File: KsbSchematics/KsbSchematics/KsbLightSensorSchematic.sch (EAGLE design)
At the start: 29 parts, among them IC1 7805L, IC2 LM311N, U1 ATTINY84

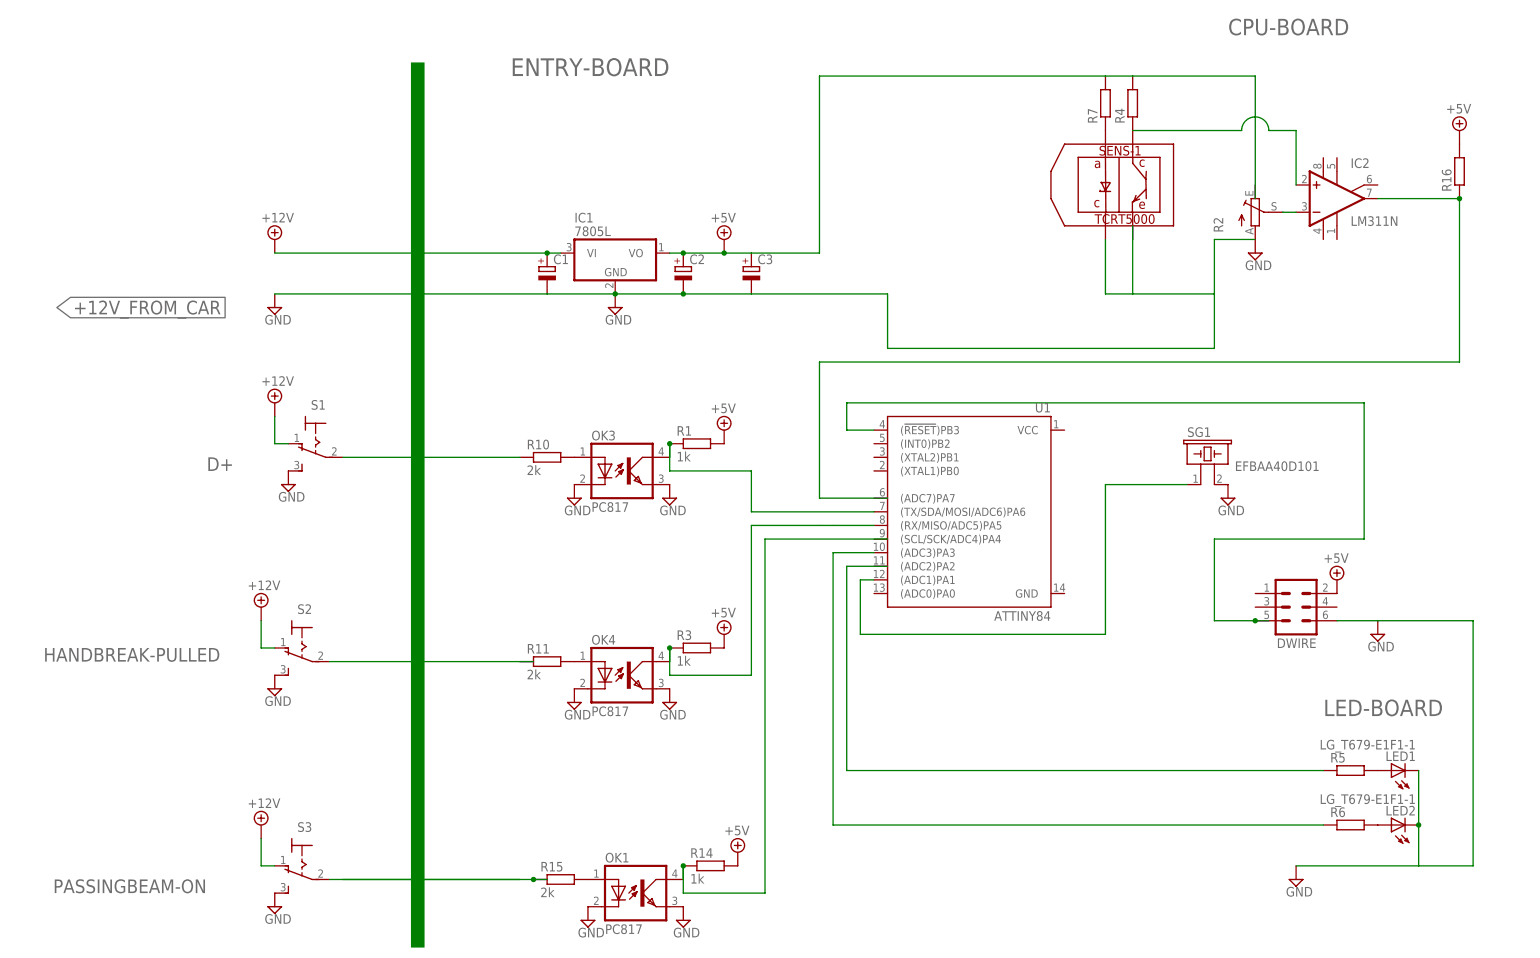
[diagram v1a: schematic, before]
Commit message: schematic changes
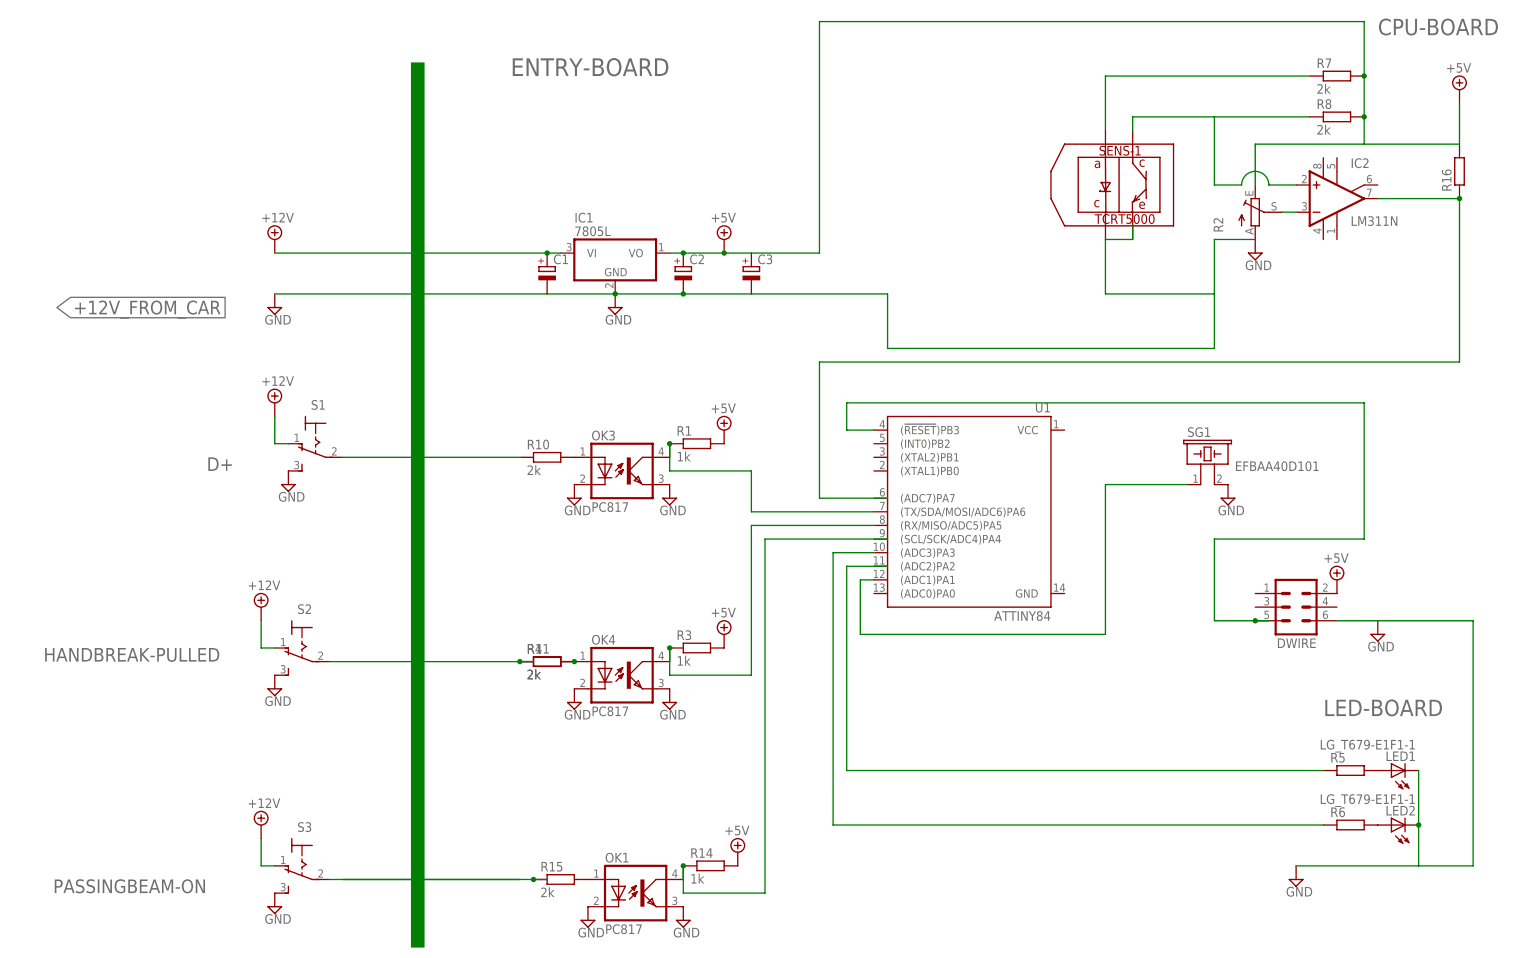
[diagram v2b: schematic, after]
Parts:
- added R8: 2k, resistor:R-EU_0613/5V
- R4, R7: value (none) -> 2k
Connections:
- net +12V: no longer R16.2
- net CPU-BOARD: now also IC2.OUT, R16.1; no longer IC2.+IN, SENS-1.P$1
- net ENTRY-BOARD: now also R16.2, R2.E, R8.2; no longer R4.2
- net N$1: now also R4.2
- net N$4: now also IC2.+IN, R8.1, SENS-1.P$1; no longer IC2.OUT, R16.1
- net PASSINGBEAM-ON: now also R4.1
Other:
- moved on the sheet: R4, R7
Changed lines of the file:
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@@
 <part name="R6" library="resistor" deviceset="R-EU_" device="0613/5V"/>
 <part name="SUPPLY17" library="supply2" deviceset="GND" device=""/>
-<part name="R4" library="resistor" deviceset="R-EU_" device="0613/5V"/>
-<part name="R7" library="resistor" deviceset="R-EU_" device="0613/5V"/>
 <part name="R10" library="resistor" deviceset="R-EU_" device="0613/5V" value="2k"/>
 <part name="R11" library="resistor" deviceset="R-EU_" device="0613/5V" value="2k"/>
@@
 <part name="DWIRE" library="con-lstb" deviceset="MA03-2" device=""/>
 <part name="SUPPLY25" library="supply2" deviceset="GND" device=""/>
+<part name="R4" library="resistor" deviceset="R-EU_" device="0613/5V" value="2k"/>
+<part name="R7" library="resistor" deviceset="R-EU_" device="0613/5V" value="2k"/>
+<part name="R8" library="resistor" deviceset="R-EU_" device="0613/5V" value="2k"/>
 </parts>
 <sheets>
@@
 <instance part="R6" gate="G$1" x="134.62" y="17.78"/>
 <instance part="SUPPLY17" gate="GND" x="111.76" y="78.74"/>
-<instance part="R4" gate="G$1" x="93.98" y="152.4" rot="R90"/>
-<instance part="R7" gate="G$1" x="88.9" y="152.4" rot="R90"/>
 <instance part="R10" gate="G$1" x="-15.24" y="86.36"/>
 <instance part="R11" gate="G$1" x="-15.24" y="48.26"/>
@@
 <instance part="R15" gate="G$1" x="-12.7" y="7.62"/>
 <instance part="R16" gate="G$1" x="154.94" y="139.7" rot="R90"/>
-<instance part="SUPPLY22" gate="+12V" x="154.94" y="147.32"/>
+<instance part="SUPPLY22" gate="+12V" x="154.94" y="154.94"/>
 <instance part="SUPPLY23" gate="+12V" x="132.08" y="63.5"/>
 <instance part="SUPPLY24" gate="GND" x="139.7" y="53.34"/>
 <instance part="DWIRE" gate="1" x="124.46" y="58.42" rot="R180"/>
 <instance part="SUPPLY25" gate="GND" x="-66.04" y="114.3"/>
+<instance part="R4" gate="G$1" x="-15.24" y="48.26"/>
+<instance part="R7" gate="G$1" x="132.08" y="157.48"/>
+<instance part="R8" gate="G$1" x="132.08" y="149.86"/>
 </instances>
 <busses>
@@
 <pinref part="R14" gate="G$1" pin="2"/>
 <pinref part="SUPPLY20" gate="+12V" pin="+12V"/>
-</segment>
-<segment>
-<pinref part="R16" gate="G$1" pin="2"/>
-<pinref part="SUPPLY22" gate="+12V" pin="+12V"/>
 </segment>
 <segment>
@@
 <wire x1="109.22" y1="116.84" x2="109.22" y2="127" width="0.1524" layer="91"/>
 <wire x1="109.22" y1="127" x2="116.84" y2="127" width="0.1524" layer="91"/>
+<pinref part="SENS-1" gate="G$1" pin="P$4"/>
+<wire x1="88.9" y1="127" x2="88.9" y2="116.84" width="0.1524" layer="91"/>
+<wire x1="109.22" y1="116.84" x2="88.9" y2="116.84" width="0.1524" layer="91"/>
 <wire x1="93.98" y1="129.54" x2="93.98" y2="127" width="0.1524" layer="91"/>
 <pinref part="SENS-1" gate="G$1" pin="P$2"/>
-<wire x1="93.98" y1="127" x2="93.98" y2="116.84" width="0.1524" layer="91"/>
-<wire x1="88.9" y1="116.84" x2="93.98" y2="116.84" width="0.1524" layer="91"/>
-<pinref part="SENS-1" gate="G$1" pin="P$4"/>
-<wire x1="88.9" y1="127" x2="88.9" y2="116.84" width="0.1524" layer="91"/>
-<wire x1="109.22" y1="116.84" x2="93.98" y2="116.84" width="0.1524" layer="91"/>
+<wire x1="88.9" y1="127" x2="93.98" y2="127" width="0.1524" layer="91"/>
 </segment>
 <segment>
@@
 </segment>
 </net>
-<net name="N$4" class="0">
+<net name="CPU-BOARD" class="0">
 <segment>
 <wire x1="154.94" y1="134.62" x2="154.94" y2="104.14" width="0.1524" layer="91"/>
@@
 <wire x1="35.56" y1="104.14" x2="35.56" y2="78.74" width="0.1524" layer="91"/>
 <wire x1="35.56" y1="78.74" x2="48.26" y2="78.74" width="0.1524" layer="91"/>
+<label x="139.7" y="165.1" size="3.048" layer="95"/>
 </segment>
 </net>
@@
 <pinref part="OK4" gate="A" pin="A"/>
 <pinref part="R11" gate="G$1" pin="2"/>
+<pinref part="R4" gate="G$1" pin="2"/>
+<junction x="-10.16" y="48.26"/>
+<pinref part="R4" gate="G$1" pin="2"/>
 </segment>
 </net>
@@
 <pinref part="S2" gate="1" pin="P"/>
 <wire x1="-20.32" y1="48.26" x2="-55.88" y2="48.26" width="0.1524" layer="91"/>
+<pinref part="R4" gate="G$1" pin="1"/>
+<junction x="-20.32" y="48.26"/>
 </segment>
 <segment>
@@
 <pinref part="SUPPLY1" gate="+12V" pin="+12V"/>
 <pinref part="C1" gate="G$1" pin="+"/>
-</segment>
-</net>
-<net name="N$2" class="0">
-<segment>
-<pinref part="R7" gate="G$1" pin="1"/>
-<pinref part="SENS-1" gate="G$1" pin="P$3"/>
 </segment>
 </net>
@@
 <pinref part="U1" gate="U1" pin="(ADC1)PA1"/>
 <wire x1="43.18" y1="63.5" x2="45.72" y2="63.5" width="0.1524" layer="91"/>
-</segment>
-</net>
-<net name="CPU-BOARD" class="0">
-<segment>
-<wire x1="114.3" y1="147.32" x2="119.38" y2="147.32" width="0.1524" layer="91" curve="-180"/>
-<wire x1="124.46" y1="147.32" x2="124.46" y2="137.16" width="0.1524" layer="91"/>
-<pinref part="IC2" gate="A" pin="+IN"/>
-<wire x1="119.38" y1="147.32" x2="124.46" y2="147.32" width="0.1524" layer="91"/>
-<pinref part="SENS-1" gate="G$1" pin="P$1"/>
-<wire x1="114.3" y1="147.32" x2="93.98" y2="147.32" width="0.1524" layer="91"/>
-<label x="111.76" y="165.1" size="3.048" layer="95"/>
 </segment>
 </net>
@@
 <wire x1="7.62" y1="124.46" x2="10.16" y2="124.46" width="0.1524" layer="91"/>
 <pinref part="IC1" gate="A1" pin="VO"/>
-<pinref part="R4" gate="G$1" pin="2"/>
-<wire x1="35.56" y1="157.48" x2="88.9" y2="157.48" width="0.1524" layer="91"/>
-<wire x1="93.98" y1="157.48" x2="88.9" y2="157.48" width="0.1524" layer="91"/>
-<pinref part="R7" gate="G$1" pin="2"/>
-<wire x1="93.98" y1="157.48" x2="116.84" y2="157.48" width="0.1524" layer="91"/>
-<wire x1="116.84" y1="157.48" x2="116.84" y2="134.62" width="0.1524" layer="91"/>
-<wire x1="35.56" y1="157.48" x2="35.56" y2="124.46" width="0.1524" layer="91"/>
+<wire x1="35.56" y1="167.64" x2="35.56" y2="124.46" width="0.1524" layer="91"/>
 <wire x1="35.56" y1="124.46" x2="22.86" y2="124.46" width="0.1524" layer="91"/>
 <label x="7.62" y="157.48" size="3.302" layer="95" rot="MR0"/>
-</segment>
-</net>
+<wire x1="35.56" y1="167.64" x2="137.16" y2="167.64" width="0.1524" layer="91"/>
+<wire x1="137.16" y1="167.64" x2="137.16" y2="157.48" width="0.1524" layer="91"/>
+<pinref part="R16" gate="G$1" pin="2"/>
+<pinref part="SUPPLY22" gate="+12V" pin="+12V"/>
+<wire x1="137.16" y1="157.48" x2="137.16" y2="149.86" width="0.1524" layer="91"/>
+<wire x1="137.16" y1="149.86" x2="137.16" y2="144.78" width="0.1524" layer="91"/>
+<wire x1="154.94" y1="152.4" x2="154.94" y2="144.78" width="0.1524" layer="91"/>
+<wire x1="137.16" y1="144.78" x2="154.94" y2="144.78" width="0.1524" layer="91"/>
+<wire x1="137.16" y1="144.78" x2="116.84" y2="144.78" width="0.1524" layer="91"/>
+<pinref part="R2" gate="1" pin="E"/>
+<wire x1="116.84" y1="144.78" x2="116.84" y2="137.16" width="0.1524" layer="91"/>
+<pinref part="R7" gate="G$1" pin="2"/>
+<junction x="137.16" y="157.48"/>
+<pinref part="R8" gate="G$1" pin="2"/>
+<junction x="137.16" y="149.86"/>
+</segment>
+</net>
+<net name="N$2" class="0">
+<segment>
+<pinref part="R7" gate="G$1" pin="1"/>
+<wire x1="127" y1="157.48" x2="88.9" y2="157.48" width="0.1524" layer="91"/>
+<pinref part="SENS-1" gate="G$1" pin="P$3"/>
+<wire x1="88.9" y1="157.48" x2="88.9" y2="147.32" width="0.1524" layer="91"/>
+</segment>
+</net>
+<net name="N$4" class="0">
+<segment>
+<pinref part="R8" gate="G$1" pin="1"/>
+<wire x1="127" y1="149.86" x2="109.22" y2="149.86" width="0.1524" layer="91"/>
+<pinref part="SENS-1" gate="G$1" pin="P$1"/>
+<wire x1="109.22" y1="149.86" x2="93.98" y2="149.86" width="0.1524" layer="91"/>
+<wire x1="93.98" y1="149.86" x2="93.98" y2="147.32" width="0.1524" layer="91"/>
+<wire x1="109.22" y1="149.86" x2="109.22" y2="137.16" width="0.1524" layer="91"/>
+<wire x1="109.22" y1="137.16" x2="114.3" y2="137.16" width="0.1524" layer="91"/>
+<pinref part="IC2" gate="A" pin="+IN"/>
+<wire x1="124.46" y1="137.16" x2="119.38" y2="137.16" width="0.1524" layer="91"/>
+<wire x1="114.3" y1="137.16" x2="119.38" y2="137.16" width="0.1524" layer="91" curve="-180"/>
+</segment>
+</net>
